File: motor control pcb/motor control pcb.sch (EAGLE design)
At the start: 81 parts, among them IC1 7805TV, IC2 A3949, IC3 SMS-12, IC4 SN75176ASOIC, IC5 ATMEGA328, IC6 FT232RL, IC7 LM358D, IC8 MAX6675, Q1 PH7030L, Q2 PH7030L, Q3 PH7030L, Q4 16MHZ, T1 BSS84, X1 9090-4V, X5 C-GRID-04-70543, X6 MSTBV10

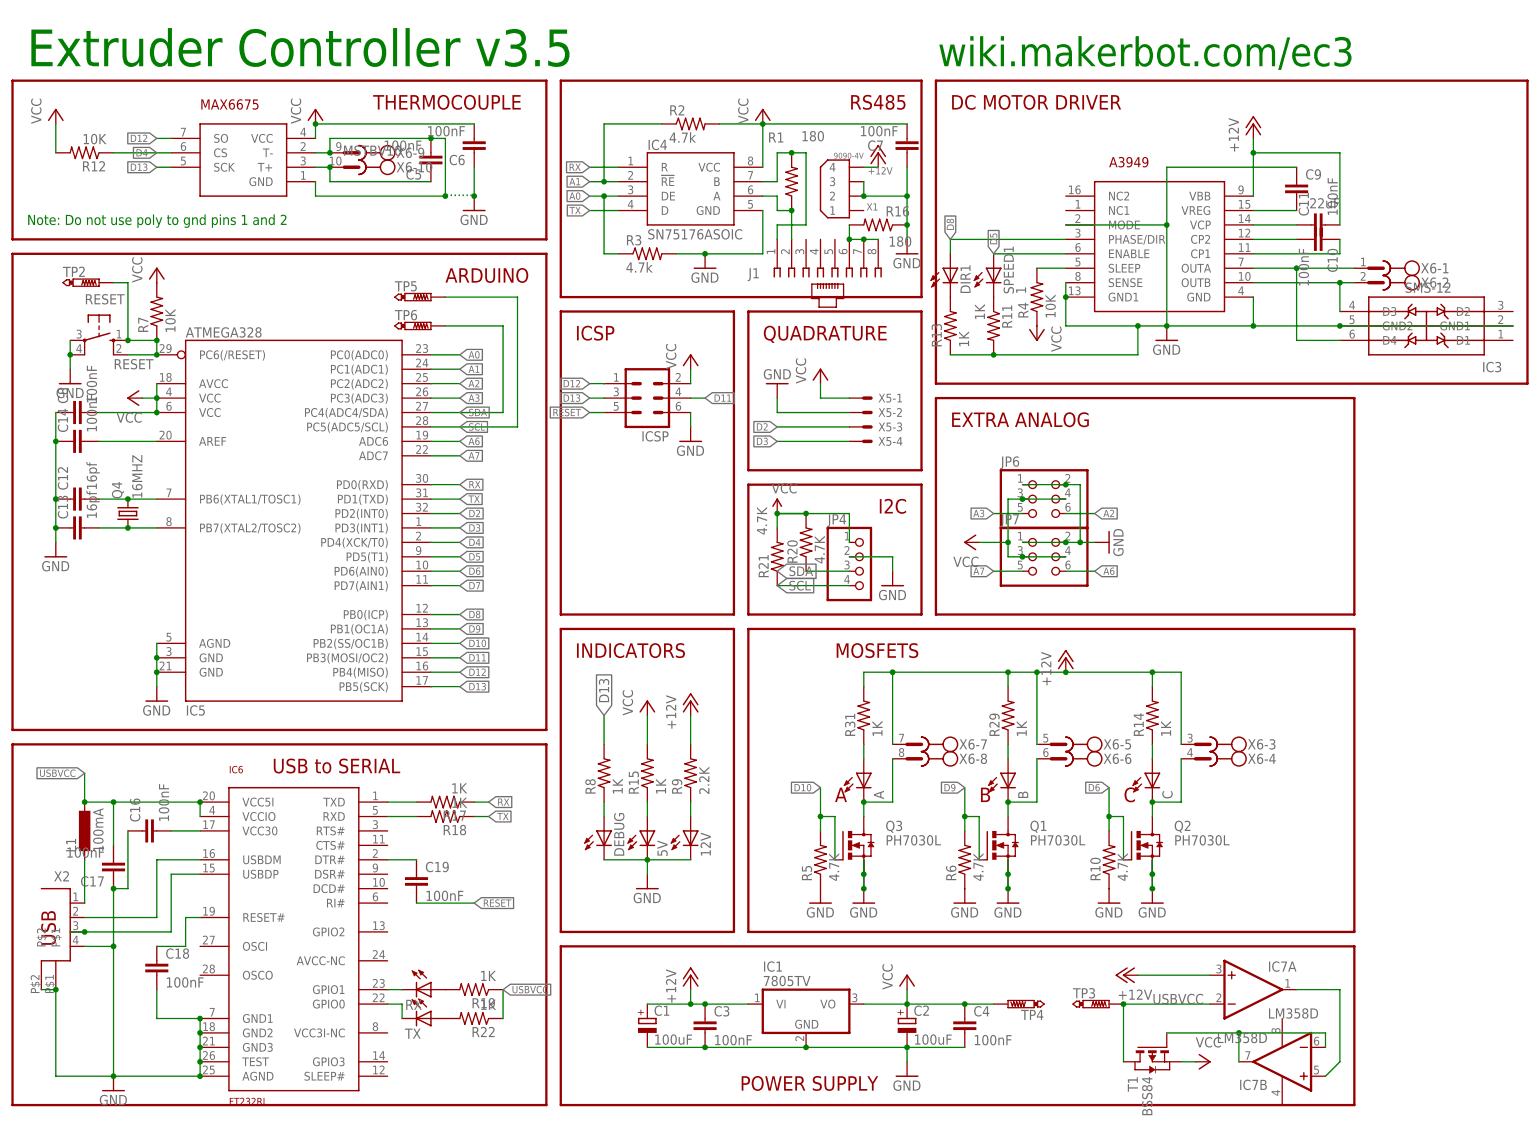
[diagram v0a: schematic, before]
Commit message: Motor control PCB
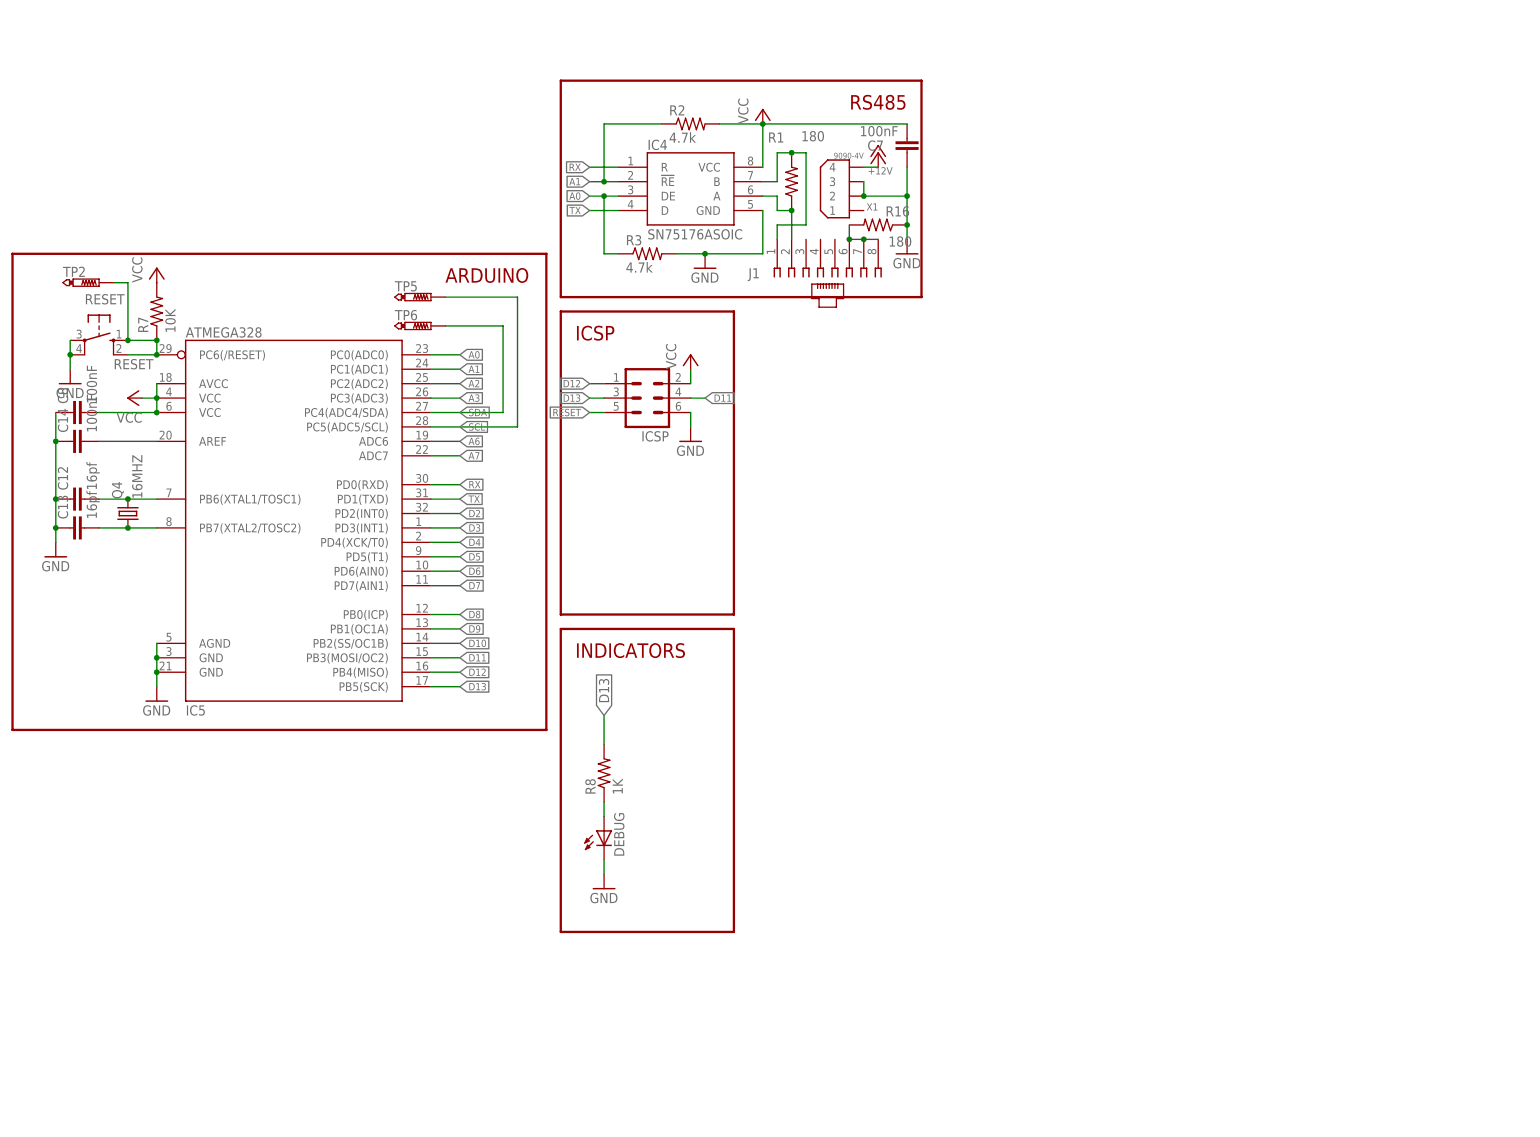
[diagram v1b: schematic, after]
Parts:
- removed 12V, 5V, A, B, C, DIR1, RX, TX: (no value), SparkFun:LED0805
- removed C1, C2: 100uF, rcl:CPOL-EUE3.5-8
- removed C10, C11, C16, C17, C18, C19, C3, C4, C5, C6: 100nF, SparkFun:CAP0805
- removed C9: .22uF, SparkFun:CAP0805
- removed IC1: 7805TV, linear:7805TV
- removed IC2: A3949, reprap:A3949
- removed IC3: SMS-12, reprap:TVS-DIODE-ARRAY
- removed IC6: FT232RL, reprap:FT232RL
- removed IC7: LM358D, linear:LM358D
- removed IC8: MAX6675, reprap:MAX6675
- removed JP4: (no value), pinhead:PINHD-1X4
- removed JP6, JP7: (no value), pinhead:PINHD-2X3
- removed L1: 100mA, resistor:L-EUL1812
- removed Q1, Q2, Q3: PH7030L, transistor-power:PH7030L
- removed R10, R20, R21, R5, R6: 4.7K, SparkFun:RESISTOR
- removed R11, R13, R14, R15, R17, R18, R19, R22, R29, R31: 1K, SparkFun:RESISTOR
- removed R12, R4: 10K, SparkFun:RESISTOR
- removed R9: 2.2K, SparkFun:RESISTOR
- removed SPEED1: 1, SparkFun:LED0805
- removed T1: BSS84, zetex:PMOSSOT23
- removed TP3, TP4: PTR1TP09R, testpad:PTR1TP09R
- removed X2: (no value), reprap:USBA
- removed X5: C-GRID-04-70543, reprap:C-GRID-04-70543
- removed X6: MSTBV10, con-phoenix-508:MSTBV10
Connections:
- removed net APWR: A.C, Q3.D, X6-8.1
- removed net BPWR: B.C, Q1.D, X6-6.1
- removed net CPWR: C.C, Q2.D, X6-4.1
- removed net N$1: C5.2, IC8.GND, IC8.T-, X6-9.1
- removed net N$11: C5.1, IC8.T+, X6-10.1
- removed net N$12: IC2.SLEEP, R4.2
- removed net N$18: R11.1, SPEED1.C
- removed net N$2: C.A, R14.1
- removed net N$23: DIR1.C, R13.2
- removed net N$25: 5V.A, R15.1
- removed net N$26: 12V.A, R9.1
- removed net N$29: IC6.USBDP, X2.3
- removed net N$3: C9.2, IC2.VREG
- removed net N$30: IC6.USBDM, X2.2
- removed net N$36: C18.1, IC6.RESET#
- removed net N$37: L1.2, X2.1
- removed net N$38: C16.2, IC6.VCC30
- removed net N$39: R19.2, RX.A
- removed net N$4: IC2.OUTA, IC3.D4, X6-1.1
- removed net N$40: R22.2, TX.A
- removed net N$41: A.A, R31.1
- removed net N$42: B.A, R29.1
- removed net N$44: IC6.GPIO1, RX.C
- removed net N$45: IC6.GPIO0, TX.C
- removed net N$46: C19.1, IC6.DTR#
- removed net N$47: IC6.TXD, R17.2
- removed net N$48: IC6.RXD, R18.2
- removed net N$5: IC2.OUTB, IC3.D3, X6-2.1
- removed net N$50: IC7A.OUT, IC7B.+IN
- removed net N$51: IC7B.-IN, IC7B.OUT, T1.G
- removed net N$6: C10.2, IC2.CP2
- removed net N$7: C10.1, IC2.CP1
- removed net N$9: C11.1, IC2.VCP
- removed net USBVCC: C17.2, IC6.VCC5I, IC6.VCCIO, IC7A.-IN, L1.1, R19.1, R22.1, T1.D, TP3.TP
- net +12V: no longer C1.+, C11.2, C3.1, IC1.VI, IC2.VBB, IC7A.+IN, R14.2, R29.2, R31.2, R9.2, X6-3.1, X6-5.1, X6-7.1
- net A2: no longer JP6.6
- net A3: no longer JP6.5
- net A6: no longer JP7.6
- net A7: no longer JP7.5
- net D10: no longer Q3.G, R5.2
- net D12: no longer IC8.SO
- net D13: no longer IC8.SCK
- net D2: no longer X5-3.S
- net D3: no longer X5-4.S
- net D4: no longer IC8.CS, R12.1
- net D5: no longer IC2.ENABLE, SPEED1.A
- net D6: no longer Q2.G, R10.2
- net D8: no longer DIR1.A, IC2.PHASE/DIR
- net D9: no longer Q1.G, R6.2
- net GND: no longer 12V.C, 5V.C, C1.-, C16.1, C17.1, C18.2, C2.-, C3.2, C4.2, C6.1, C9.1, IC1.GND, IC2.GND, IC2.GND1, IC2.MODE, IC2.SENSE, IC3.GND1, IC3.GND2, IC6.AGND, IC6.GND1, IC6.GND2, IC6.GND3, IC6.TEST, JP4.2, JP6.1, JP6.2, JP7.1, JP7.2, Q1.S, Q1.S@1, Q1.S@2, Q2.S, Q2.S@1, Q2.S@2, Q3.S, Q3.S@1, Q3.S@2, R10.1, R11.2, R13.1, R5.1, R6.1, X2.4, X2.P$1, X2.P$2, X5-2.S
- net RESET: no longer C19.2
- net RX: no longer R17.1
- net SCL: no longer JP4.4, R21.1
- net SDA: no longer JP4.3, R20.1
- net TX: no longer R18.1
- net VCC: no longer C2.+, C4.1, C6.2, IC1.VO, IC8.VCC, JP4.1, JP6.3, JP6.4, JP7.3, JP7.4, R12.2, R15.2, R20.2, R21.2, R4.1, T1.S, TP4.TP, X5-1.S
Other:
- note removed: "......."
- note removed: "A"
- note removed: "B"
- note removed: "C"
- note removed: "DC MOTOR DRIVER"
- note removed: "EXTRA ANALOG"
- note removed: "Extruder Controller v3.5"
- note removed: "I2C"
- note removed: "MOSFETS"
- note removed: "Note: Do not use poly to gnd pins 1 and 2"
- note removed: "POWER SUPPLY"
- note removed: "QUADRATURE"
- note removed: "THERMOCOUPLE"
- note removed: "USB to SERIAL"
- note removed: "wiki.makerbot.com/ec3"
